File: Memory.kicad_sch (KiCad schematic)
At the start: 13 parts, among them IC1 SDRAM_IS42S16320F-7TL, U2 NAND_MT29F2G16ABAEAWP-AITE

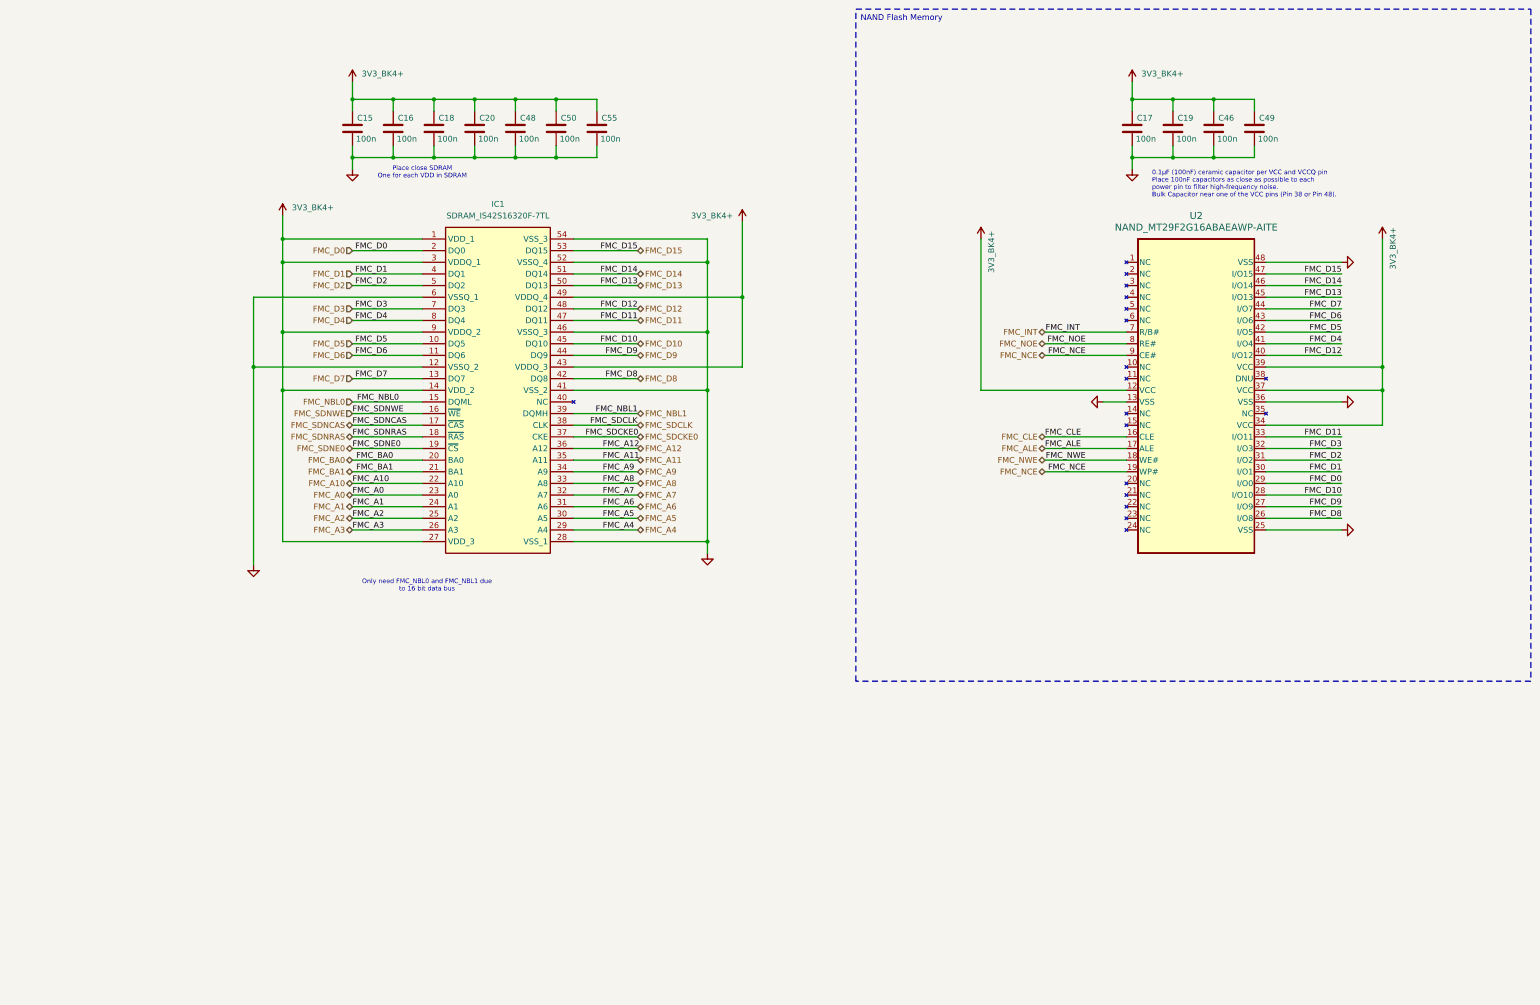
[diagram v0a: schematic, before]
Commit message: Update
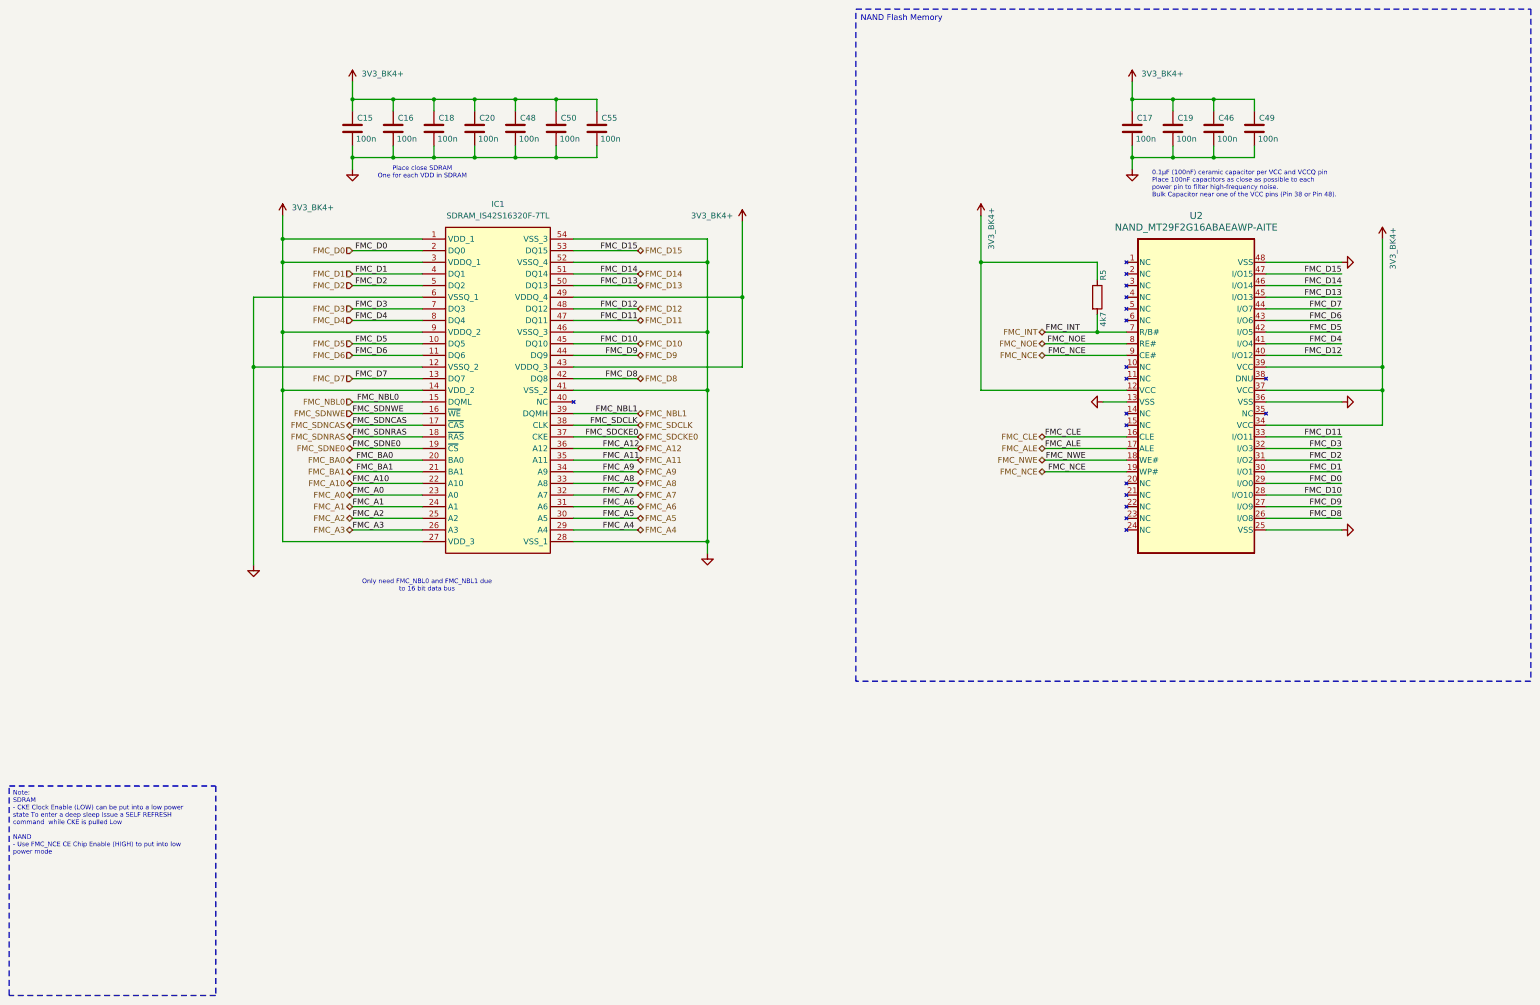
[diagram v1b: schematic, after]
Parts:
- added R5: 4k7, Resistor_SMD:R_0805_2012Metric_1, symbol Device:R
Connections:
- net 3V3_BK4+: now also R5.1
- net FMC_INT: now also R5.2
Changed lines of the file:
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@@
 	)
 	(junction
+		(at 265.43 125.73)
+		(diameter 0)
+		(color 0 0 0 0)
+	)
+	(junction
 		(at 281.94 74.93)
 		(diameter 0)
@@
 	)
 	(junction
+		(at 240.03 110.49)
+		(diameter 0)
+		(color 0 0 0 0)
+	)
+	(junction
 		(at 120.65 87.63)
 		(diameter 0)
@@
 	(wire
 		(pts
+			(xy 265.43 110.49) (xy 240.03 110.49)
+		)
+		(stroke
+			(width 0)
+			(type default)
+		)
+	)
+	(wire
+		(pts
 			(xy 111.76 87.63) (xy 120.65 87.63)
 		)
@@
 	(wire
 		(pts
+			(xy 265.43 121.92) (xy 265.43 125.73)
+		)
+		(stroke
+			(width 0)
+			(type default)
+		)
+	)
+	(wire
+		(pts
 			(xy 151.13 110.49) (xy 180.34 110.49)
 		)
@@
 	(wire
 		(pts
+			(xy 265.43 125.73) (xy 254 125.73)
+		)
+		(stroke
+			(width 0)
+			(type default)
+		)
+	)
+	(wire
+		(pts
 			(xy 120.65 85.09) (xy 120.65 87.63)
 		)
@@
 	(wire
 		(pts
-			(xy 271.78 125.73) (xy 254 125.73)
+			(xy 271.78 125.73) (xy 265.43 125.73)
 		)
 		(stroke
@@
 	(wire
 		(pts
-			(xy 240.03 138.43) (xy 240.03 105.41)
+			(xy 240.03 138.43) (xy 240.03 110.49)
 		)
 		(stroke
@@
 	(wire
 		(pts
+			(xy 240.03 110.49) (xy 240.03 100.33)
+		)
+		(stroke
+			(width 0)
+			(type default)
+		)
+	)
+	(wire
+		(pts
 			(xy 118.11 130.81) (xy 102.87 130.81)
 		)
@@
 	(wire
 		(pts
+			(xy 265.43 114.3) (xy 265.43 110.49)
+		)
+		(stroke
+			(width 0)
+			(type default)
+		)
+	)
+	(wire
+		(pts
 			(xy 271.78 156.21) (xy 254 156.21)
 		)
@@
 		)
 	)
+	(text_box "Note:\nSDRAM\n- CKE Clock Enable (LOW) can be put into a low power state To enter a deep sleep Issue a SELF REFRESH command  while CKE is pulled Low\n\nNAND\n- Use FMC_NCE CE Chip Enable (HIGH) to put into low power mode"
+		(exclude_from_sim no)
+		(at 27.94 224.79 0)
+		(size 45.085 45.72)
+		(stroke
+			(width 0)
+			(type dash)
+		)
+		(fill
+			(type none)
+		)
+		(effects
+			(font
+				(size 1 1)
+			)
+			(justify left top)
+		)
+	)
 	(text_box "NAND Flash Memory"
 		(exclude_from_sim no)
@@
 	(symbol
 		(lib_id "power:+3.3V")
-		(at 240.03 105.41 0)
+		(at 240.03 100.33 0)
 		(mirror y)
 		(unit 1)
@@
 		(dnp no)
 		(property "Reference" "#PWR065"
-			(at 240.03 109.22 0)
+			(at 240.03 104.14 0)
 			(effects
 				(font
@@
 		)
 		(property "Value" "3V3_BK4+"
-			(at 242.316 108.204 90)
+			(at 242.316 103.124 90)
 			(effects
 				(font
@@
 		)
 		(property "Footprint" ""
-			(at 240.03 105.41 0)
+			(at 240.03 100.33 0)
 			(effects
 				(font
@@
 		)
 		(property "Datasheet" ""
-			(at 240.03 105.41 0)
+			(at 240.03 100.33 0)
 			(effects
 				(font
@@
 		)
 		(property "Description" "Power symbol creates a global label with name \"+3.3V\""
-			(at 240.03 105.41 0)
+			(at 240.03 100.33 0)
 			(effects
 				(font
@@
 					(unit 1)
 				)
+			)
+		)
+	)
+	(symbol
+		(lib_id "Device:R")
+		(at 265.43 118.11 0)
+		(unit 1)
+		(exclude_from_sim no)
+		(in_bom yes)
+		(on_board yes)
+		(dnp no)
+		(property "Reference" "R5"
+			(at 266.7 113.284 90)
+			(effects
+				(font
+					(size 1.27 1.27)
+				)
+			)
+		)
+		(property "Value" "4k7"
+			(at 266.7 122.936 90)
+			(effects
+				(font
+					(size 1.27 1.27)
+				)
+			)
+		)
+		(property "Footprint" "Resistor_SMD:R_0805_2012Metric_1"
+			(at 263.652 118.11 90)
+			(effects
+				(font
+					(size 1.27 1.27)
+				)
+				(hide yes)
+			)
+		)
+		(property "Datasheet" "~"
+			(at 265.43 118.11 0)
+			(effects
+				(font
+					(size 1.27 1.27)
+				)
+				(hide yes)
+			)
+		)
+		(property "Description" "Resistor"
+			(at 265.43 118.11 0)
+			(effects
+				(font
+					(size 1.27 1.27)
+				)
+				(hide yes)
+			)
+		)
+		(pin "1"
+		)
+		(pin "2"
+		)
+		(instances
+			(project "STM32H7_Board"
+				(path "/9b48e30a-b912-4658-a133-1a15707d5b7d/c1273a5b-dc13-48da-a35d-ed40e44ccc48"
+					(reference "R5")
+					(unit 1)
+				)

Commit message: Update
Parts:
- C15, C16, C17, C18, C19, C20, C46, C48, C49, C50, C55: footprint Capacitor_SMD:C_0805_2012Metric -> Capacitor_SMD:C_0603_1608Metric
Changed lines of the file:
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@@
 			)
 		)
-		(property "Footprint" "Capacitor_SMD:C_0805_2012Metric"
+		(property "Footprint" "Capacitor_SMD:C_0603_1608Metric"
 			(at 282.9052 85.09 0)
 			(effects
@@
 			)
 		)
-		(property "Footprint" "Capacitor_SMD:C_0805_2012Metric"
+		(property "Footprint" "Capacitor_SMD:C_0603_1608Metric"
 			(at 148.2852 85.09 0)
 			(effects
@@
 			)
 		)
-		(property "Footprint" "Capacitor_SMD:C_0805_2012Metric"
+		(property "Footprint" "Capacitor_SMD:C_0603_1608Metric"
 			(at 300.6852 85.09 0)
 			(effects
@@
 			)
 		)
-		(property "Footprint" "Capacitor_SMD:C_0805_2012Metric"
+		(property "Footprint" "Capacitor_SMD:C_0603_1608Metric"
 			(at 112.7252 85.09 0)
 			(effects
@@
 			)
 		)
-		(property "Footprint" "Capacitor_SMD:C_0805_2012Metric"
+		(property "Footprint" "Capacitor_SMD:C_0603_1608Metric"
 			(at 157.1752 85.09 0)
 			(effects
@@
 			)
 		)
-		(property "Footprint" "Capacitor_SMD:C_0805_2012Metric"
+		(property "Footprint" "Capacitor_SMD:C_0603_1608Metric"
 			(at 103.8352 85.09 0)
 			(effects
@@
 			)
 		)
-		(property "Footprint" "Capacitor_SMD:C_0805_2012Metric"
+		(property "Footprint" "Capacitor_SMD:C_0603_1608Metric"
 			(at 274.0152 85.09 0)
 			(effects
@@
 			)
 		)
-		(property "Footprint" "Capacitor_SMD:C_0805_2012Metric"
+		(property "Footprint" "Capacitor_SMD:C_0603_1608Metric"
 			(at 139.3952 85.09 0)
 			(effects
@@
 			)
 		)
-		(property "Footprint" "Capacitor_SMD:C_0805_2012Metric"
+		(property "Footprint" "Capacitor_SMD:C_0603_1608Metric"
 			(at 121.6152 85.09 0)
 			(effects
@@
 			)
 		)
-		(property "Footprint" "Capacitor_SMD:C_0805_2012Metric"
+		(property "Footprint" "Capacitor_SMD:C_0603_1608Metric"
 			(at 291.7952 85.09 0)
 			(effects
@@
 			)
 		)
-		(property "Footprint" "Capacitor_SMD:C_0805_2012Metric"
+		(property "Footprint" "Capacitor_SMD:C_0603_1608Metric"
 			(at 130.5052 85.09 0)
 			(effects

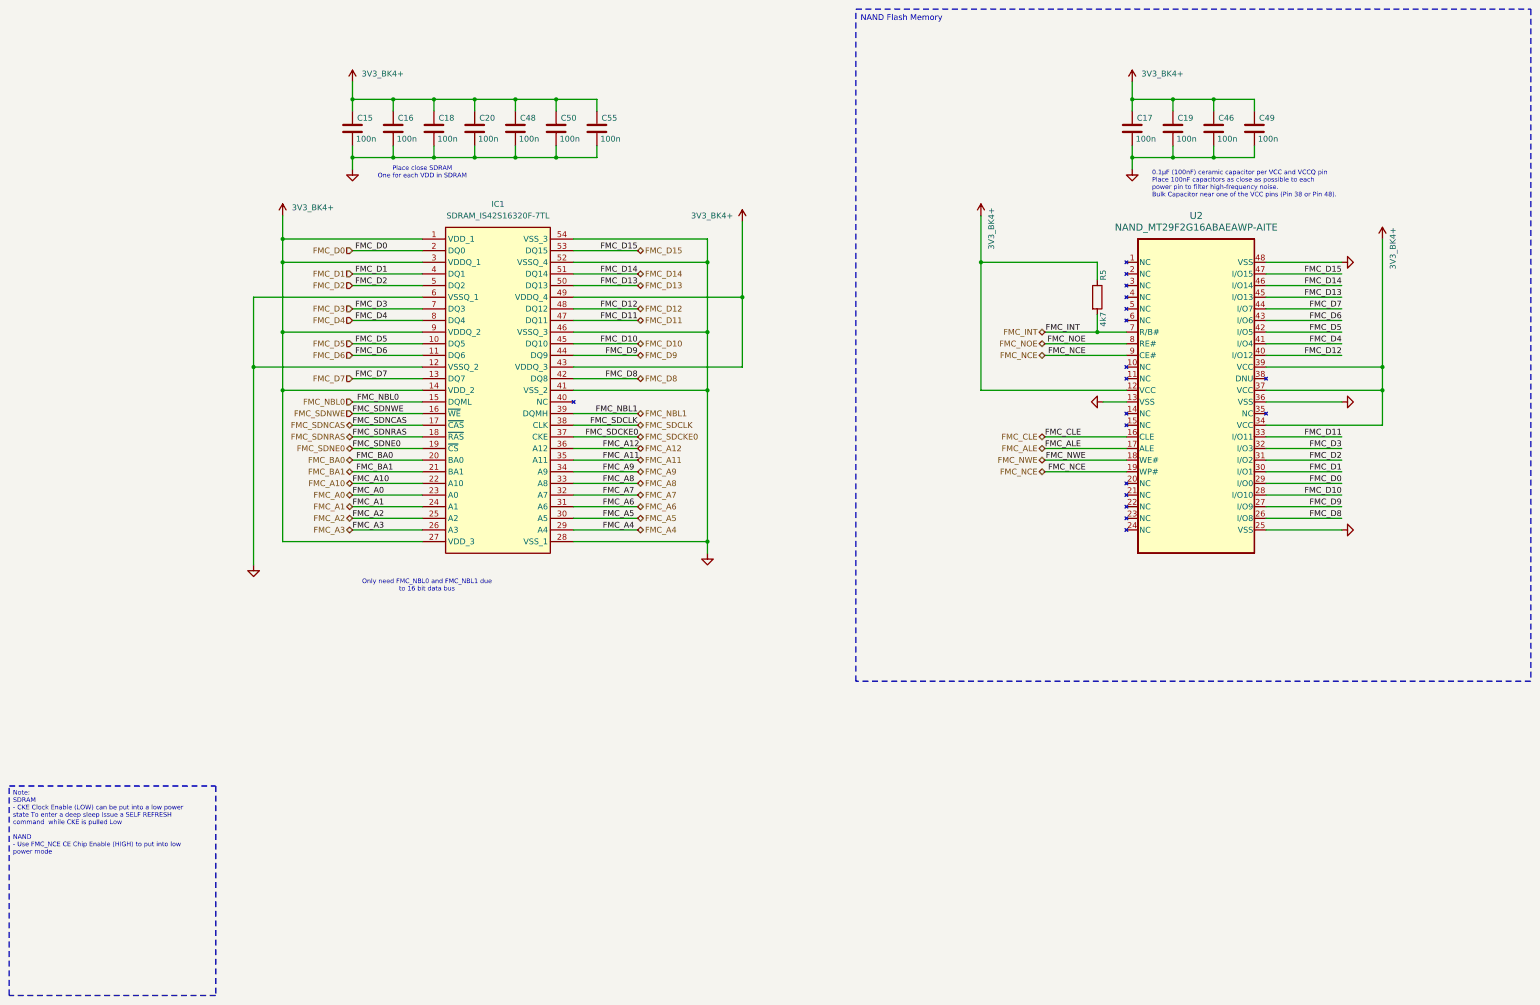
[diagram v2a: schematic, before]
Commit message: Update
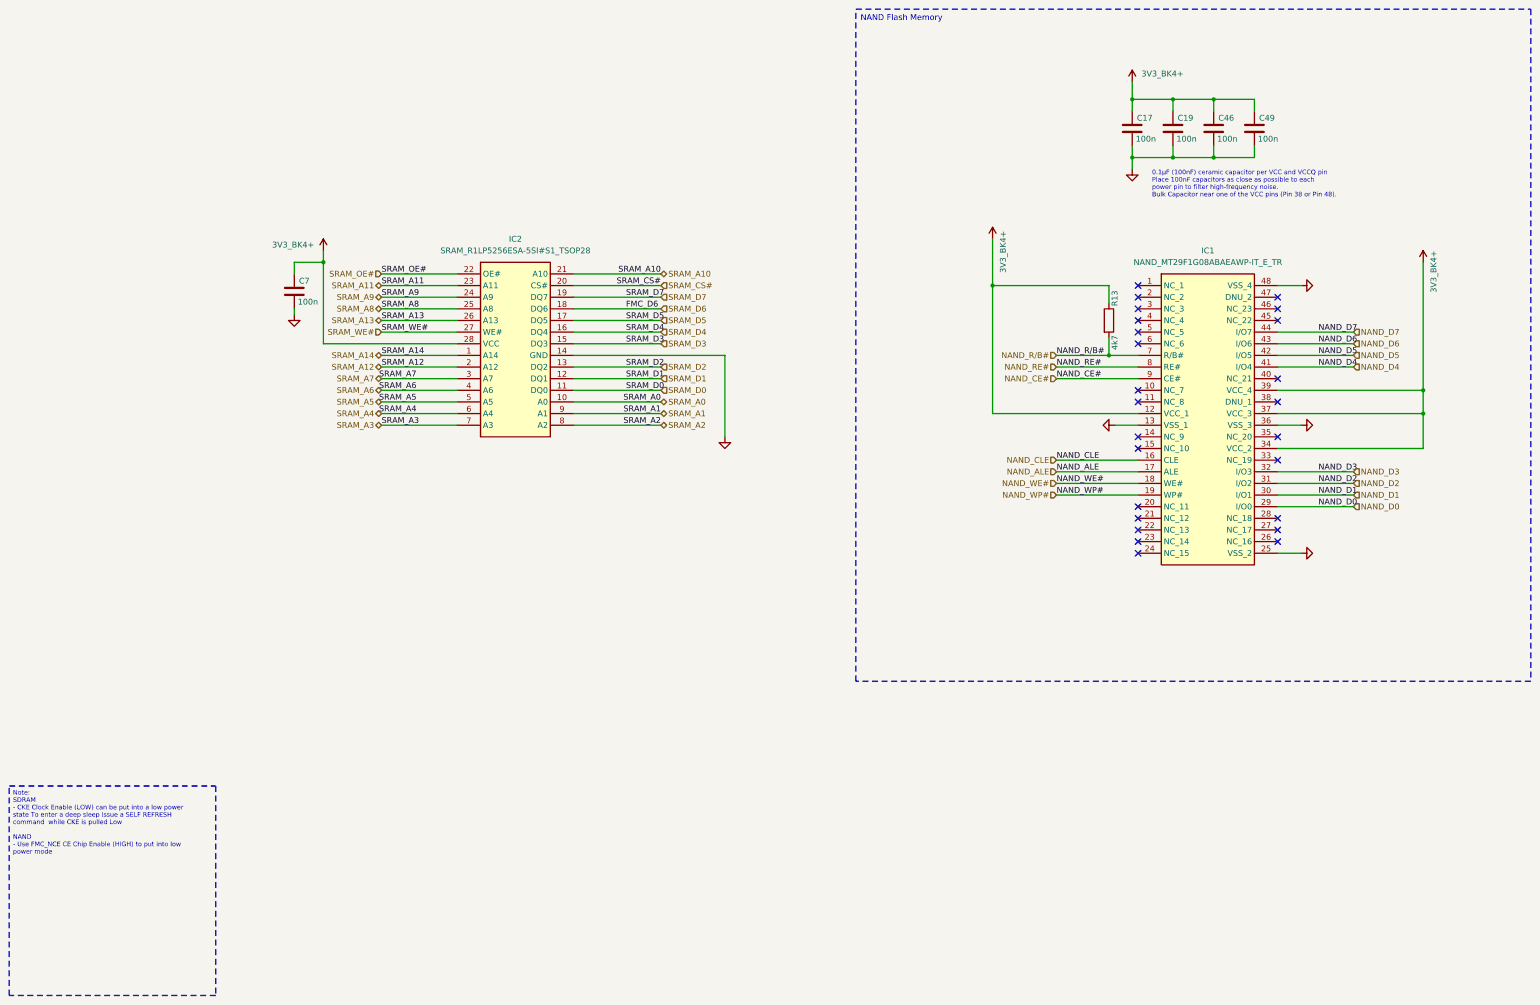
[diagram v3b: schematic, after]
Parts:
- removed C15, C16, C18, C20, C48, C50, C55: 100n, Capacitor_SMD:C_0603_1608Metric, symbol Device:C
- removed IC1: SDRAM_IS42S16320F-7TL, Personal_Project:SDRAM_IS42S16320F-6TL, symbol Personal_Projects:SDRAM_IS42S16320F-6TL
- removed R5: 4k7, Resistor_SMD:R_0805_2012Metric_1, symbol Device:R
- removed U2: NAND_MT29F2G16ABAEAWP-AITE, Personal_Project:NAND_MT29F2G16ABAEAWP-AITE_TSOP-I-48_18.4x12mm_P0.5mmNA, symbol Personal_Projects:NAND_MT29F2G16ABAEAWP-AITE.kicad_sym
- added C7: 100n, Capacitor_SMD:C_0603_1608Metric, symbol Device:C
- added IC1: NAND_MT29F1G08ABAEAWP-IT_E_TR, Personal_Project:NAND_MT29F1G08ABAEAWP-IT_E_TR_SOP50P2000X120-48N, symbol Personal_Projects:NAND_MT29F1G08ABAEAWP-IT_E_TR
- added IC2: SRAM_R1LP5256ESA-5SI#S1_TSOP28, Personal_Project:SRAM_R1LV5256ESA5SIS1_TSOP28, symbol Personal_Projects:SRAM_R1LP5256ESA-5SI#S1_TSOP28
- added R13: 4k7, Resistor_SMD:R_0805_2012Metric_1, symbol Device:R
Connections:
- net 3V3_BK4+: now also C7.1, IC1.12 (VCC_1), IC1.34 (VCC_2), IC1.37 (VCC_3), IC1.39 (VCC_4), IC2.28 (VCC), R13.1
- net GND: now also C7.2, IC1.13 (VSS_1), IC1.25 (VSS_2), IC1.36 (VSS_3), IC1.48 (VSS_4), IC2.14 (GND)
- new net NAND_ALE: IC1.17 (ALE)
- new net NAND_CE#: IC1.9 (CE#)
- new net NAND_CLE: IC1.16 (CLE)
- new net NAND_D0: IC1.29 (I/O0)
- new net NAND_D1: IC1.30 (I/O1)
- new net NAND_D2: IC1.31 (I/O2)
- new net NAND_D3: IC1.32 (I/O3)
- new net NAND_D4: IC1.41 (I/O4)
- new net NAND_D5: IC1.42 (I/O5)
- new net NAND_D6: IC1.43 (I/O6)
- new net NAND_D7: IC1.44 (I/O7)
- new net NAND_RE#: IC1.8 (RE#)
- new net NAND_R/B#: IC1.7 (R/B#), R13.2
- new net NAND_WE#: IC1.18 (WE#)
- new net NAND_WP#: IC1.19 (WP#)
- new net SRAM_A0: IC2.10 (A0)
- new net SRAM_A1: IC2.9 (A1)
- new net SRAM_A10: IC2.21 (A10)
- new net SRAM_A11: IC2.23 (A11)
- new net SRAM_A12: IC2.2 (A12)
- new net SRAM_A13: IC2.26 (A13)
- new net SRAM_A14: IC2.1 (A14)
- new net SRAM_A2: IC2.8 (A2)
- new net SRAM_A3: IC2.7 (A3)
- new net SRAM_A4: IC2.6 (A4)
- new net SRAM_A5: IC2.5 (A5)
- new net SRAM_A6: IC2.4 (A6)
- new net SRAM_A7: IC2.3 (A7)
- new net SRAM_A8: IC2.25 (A8)
- new net SRAM_A9: IC2.24 (A9)
- new net SRAM_CS#: IC2.20 (CS#)
- new net SRAM_D0: IC2.11 (DQ0)
- new net SRAM_D1: IC2.12 (DQ1)
- new net SRAM_D2: IC2.13 (DQ2)
- new net SRAM_D3: IC2.15 (DQ3)
- new net SRAM_D4: IC2.16 (DQ4)
- new net SRAM_D5: IC2.17 (DQ5)
- new net SRAM_D6: IC2.18 (DQ6)
- new net SRAM_D7: IC2.19 (DQ7)
- new net SRAM_OE#: IC2.22 (OE#)
- new net SRAM_WE#: IC2.27 (WE#)
- no-connect marks 0 -> 25
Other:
- note removed: "Only need FMC_NBL0 and FMC_NBL1 due to 16 bit data bus"
- note removed: "Place close SDRAM One for each VDD in SDRAM"
